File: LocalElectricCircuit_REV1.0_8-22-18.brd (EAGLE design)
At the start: 160 x 100 mm, 68 parts, among them IC1 PIC32MX360F512L, U1 ADS1118, U2 ADS1118, X2 MALE_VGA

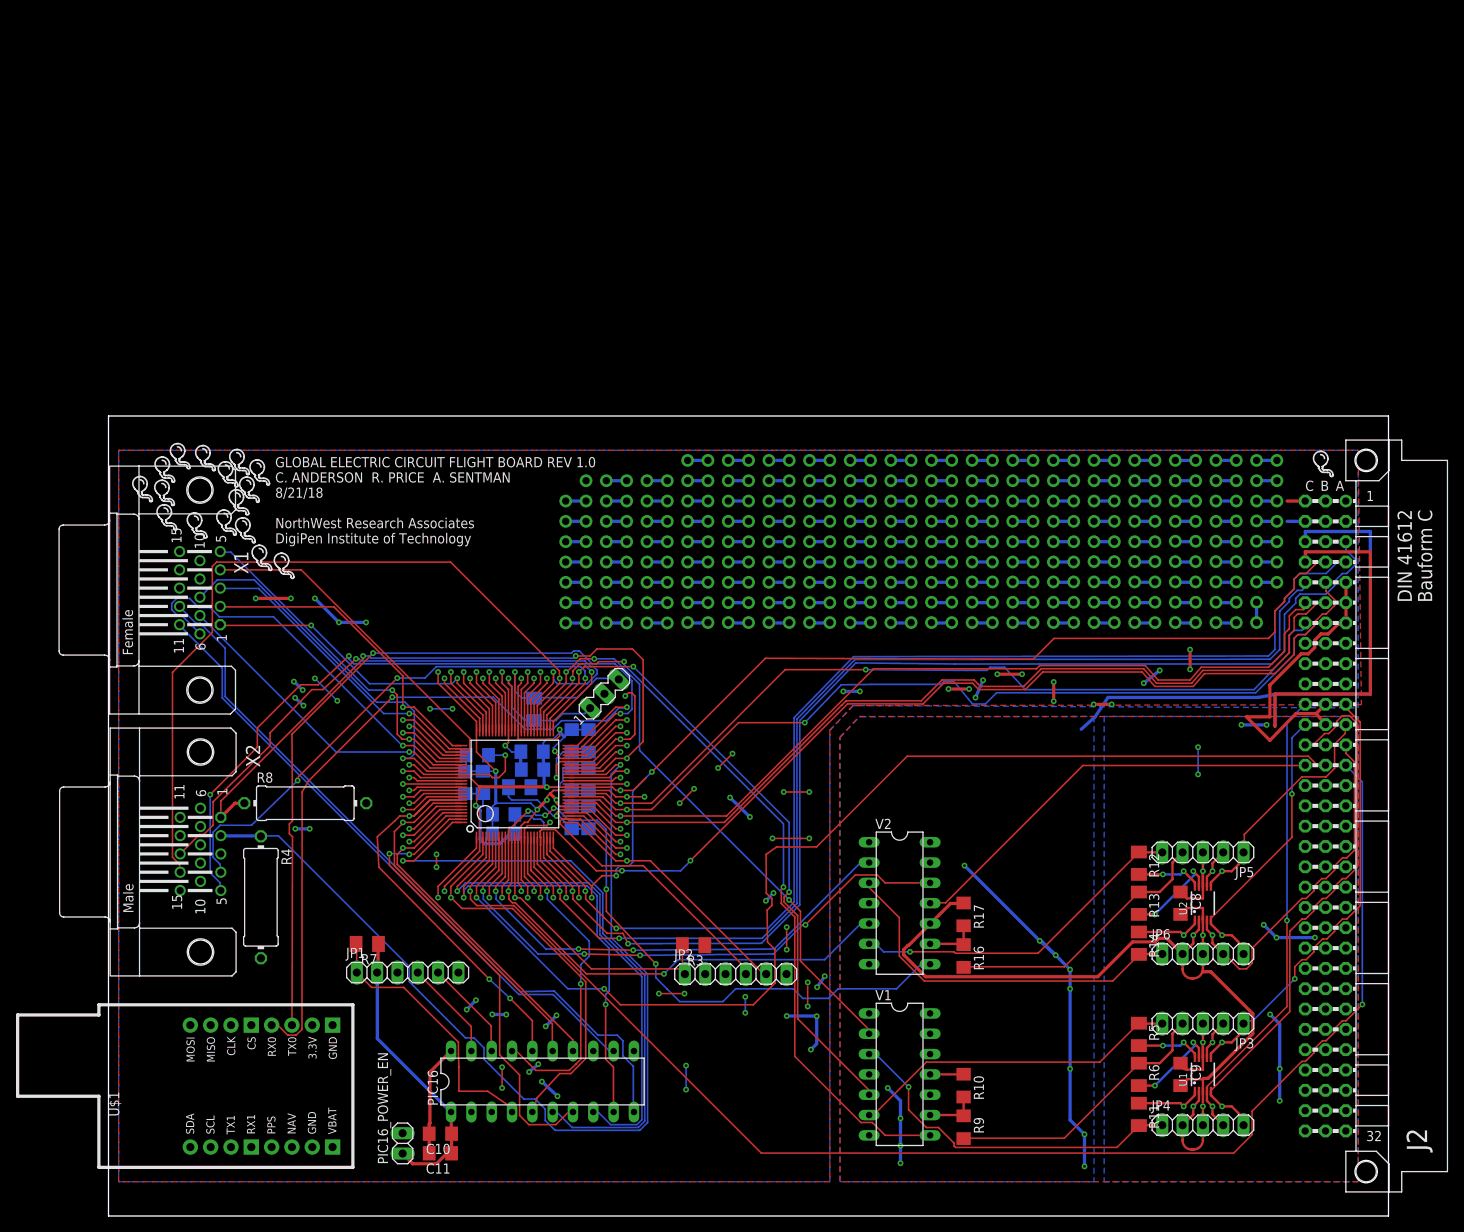
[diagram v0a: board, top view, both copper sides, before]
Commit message: THIS IS THE VERSION OF THE BOARD SENT TO BE MADE
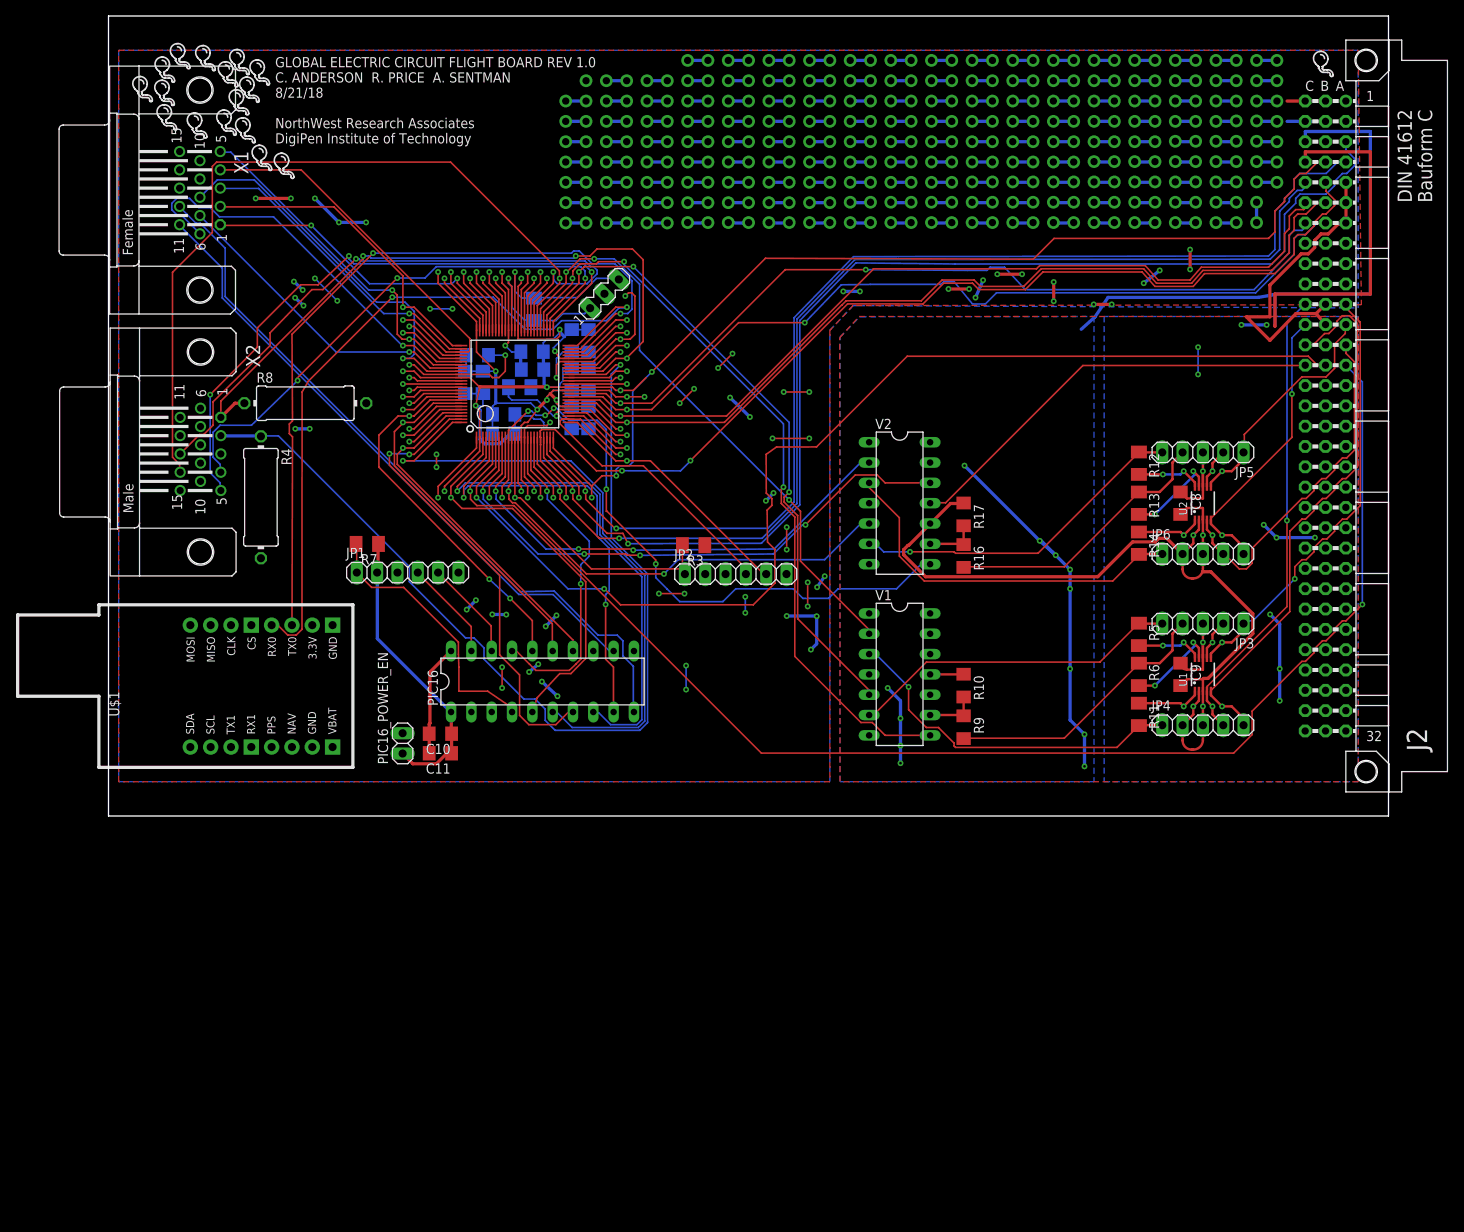
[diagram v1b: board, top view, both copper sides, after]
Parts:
- moved U$11 50.0 mm to (6.91, 87.8)
- moved U$15 50.0 mm to (14.6, 93.1)
- moved U$19 50.0 mm to (15.9, 89.6)
- moved C1 50.0 mm to (44.6, 54.2)
- moved C10 50.0 mm to (41.5, 10.3)
- moved C11 50.0 mm to (41.5, 7.84)
- moved C12 50.0 mm to (57.9, 59.4)
- moved C13 50.0 mm to (49.4, 50.2)
- moved C14 50.0 mm to (57.9, 54.6)
- moved C15 50.0 mm to (46.8, 54.2)
- moved C16 50.0 mm to (53.0, 55.8)
- moved C17 50.0 mm to (57.9, 49.8)
- moved C2 50.0 mm to (49.4, 47.8)
- moved C3 50.0 mm to (60.0, 49.8)
- moved C4 50.0 mm to (60.0, 59.4)
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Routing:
- net N$79: track 7.43 -> 0.00 mm
